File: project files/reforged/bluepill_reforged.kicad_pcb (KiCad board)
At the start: 2 copper layers, 53.3 x 22.9 mm, 38 parts, among them J1 USB_C_Receptacle_USB2.0, J2 Left Castellation, J3 STDC14, J4 Right Castellation, SW1 Boot0, SW2 Reset, U1 AMS1117-3.3, U2 STM32F103C8Tx, Y1 8MHz, Y2 32768Hz

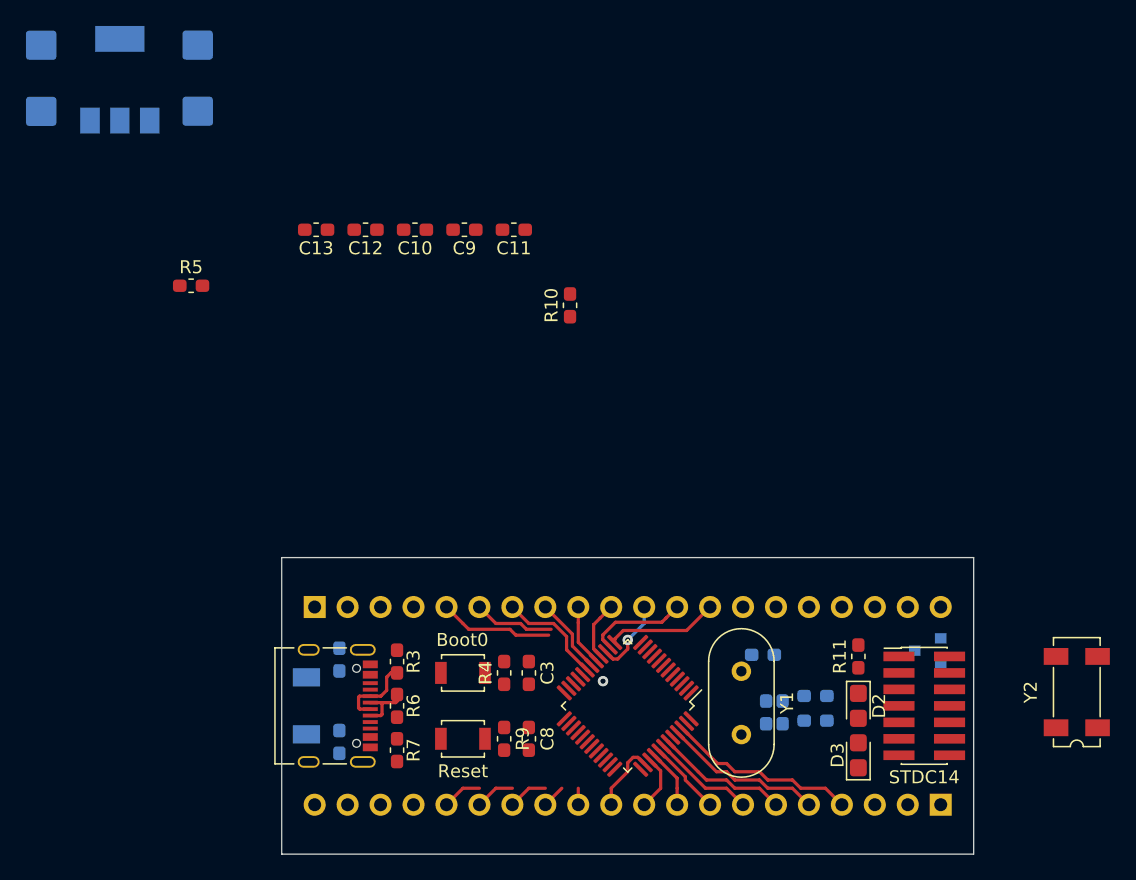
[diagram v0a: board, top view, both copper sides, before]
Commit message: minor
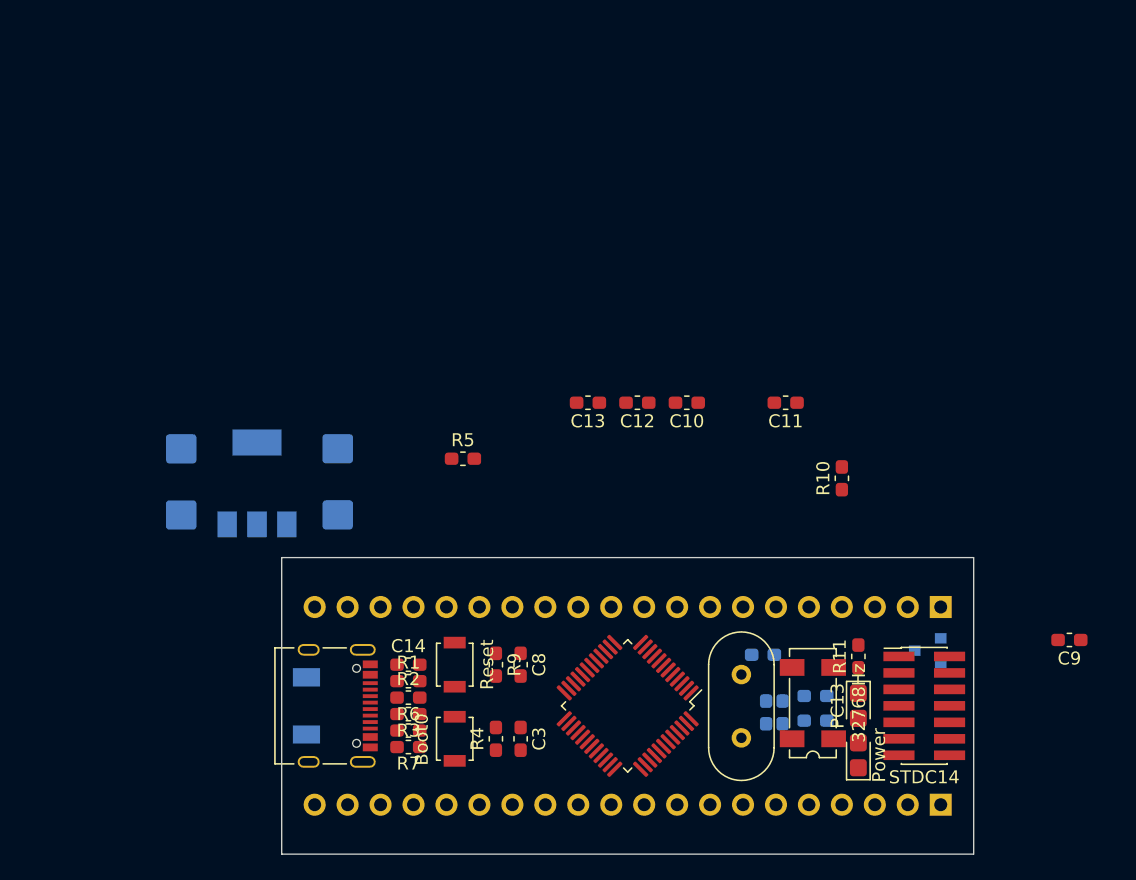
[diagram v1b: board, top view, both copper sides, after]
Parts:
- added C14: 100n, Capacitor_SMD:C_0603_1608Metric_Pad1.05x0.95mm_HandSolder, F.Cu at (138.0, 135.3)
- R1, R2: moved to F.Cu
- moved C9 56.3 mm to (189.0, 133.3)
- moved J4 48.3 mm to (179.1, 130.8), turned to 90 degrees
- moved C1 32.9 mm to (120.5, 121.2)
- moved C2 32.9 mm to (132.6, 121.2)
- moved U1 32.9 mm to (126.4, 121.3)
- moved R5 24.8 mm to (142.2, 119.4)
- moved C10 24.8 mm to (159.5, 115.1)
- moved C11 24.8 mm to (167.1, 115.1)
- moved C12 24.8 mm to (155.7, 115.1)
- moved C13 24.8 mm to (151.9, 115.1)
- moved R10 24.8 mm to (171.4, 120.9)
- moved Y2 20.4 mm to (169.2, 138.2)
- moved R2 6.32 mm to (138.0, 137.8), turned to 0 degrees
- moved SW2 5.75 mm to (141.6, 135.3), turned to 90 degrees
- moved C8 5.75 mm to (146.7, 135.3)
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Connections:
- J4 pad 1: GNDREF -> +BATT
- J4 pad 10: PA6 -> PA5
- J4 pad 11: PA5 -> PA6
- J4 pad 12: PA4 -> PA7
- J4 pad 13: PA3 -> PB0
- J4 pad 14: PA2 -> PB1
- J4 pad 15: PA1 -> PB10
- J4 pad 16: PA0 -> PB11
- J4 pad 17: PC15 -> NRST
- J4 pad 18: PC14 -> +3V3
- J4 pad 19: PC13 -> GNDREF
- J4 pad 2: GNDREF -> PC13
- J4 pad 20: +BATT -> GNDREF
- J4 pad 3: +3V3 -> PC14
- J4 pad 4: NRST -> PC15
- J4 pad 5: PB11 -> PA0
- J4 pad 6: PB10 -> PA1
- J4 pad 7: PB1 -> PA2
- J4 pad 8: PB0 -> PA3
- J4 pad 9: PA7 -> PA4
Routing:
- net PB9: track 14.8 -> 0.00 mm
- net PB8: track 12.4 -> 0.00 mm
- net PB7: track 10.4 -> 0.00 mm
- net PB11: track 8.81 -> 0.00 mm
- net PA3: track 8.64 -> 0.00 mm
- net PB1: track 8.38 -> 0.00 mm
- net PB6: track 8.02 -> 0.00 mm
- net PA4: track 7.79 -> 0.00 mm
- net PB10: track 6.24 -> 0.00 mm
- net D-: track 6.11 -> 0.00 mm
- net PA5: track 6.02 -> 0.00 mm, vias 1 -> 0
- net PB0: track 5.98 -> 0.00 mm
- net PB5: track 5.80 -> 0.00 mm
- net PA15: track 5.52 -> 0.00 mm
- net PA7: track 4.72 -> 0.00 mm
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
